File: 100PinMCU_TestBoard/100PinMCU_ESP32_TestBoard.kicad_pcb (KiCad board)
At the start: 4 copper layers, 117.6 x 50.6 mm, 120 parts, among them IC1 TCAN3413DR, IC2 TCAN3413DR, J1 ADC_Breakout, J10 SWD_PinHeader, J2 LogicAnalyzer_1, J3 CAN_1, J4 CAN_2, J5 LogicAnalyzer_2, J6 CAN_Breakout, J7 USB_C_Receptacle_USB2.0_16P, J8 SWD_Header_02x02, J9 USB_C_Receptacle_USB2.0_16P, SW1 BOOT Switch, SW2 RESET Button, U1 ESP32-C6-MINI-1, U2 MCP1826S, U3 STM32G491VET6, U4 TPS2117DRLR, Y1 Crystal

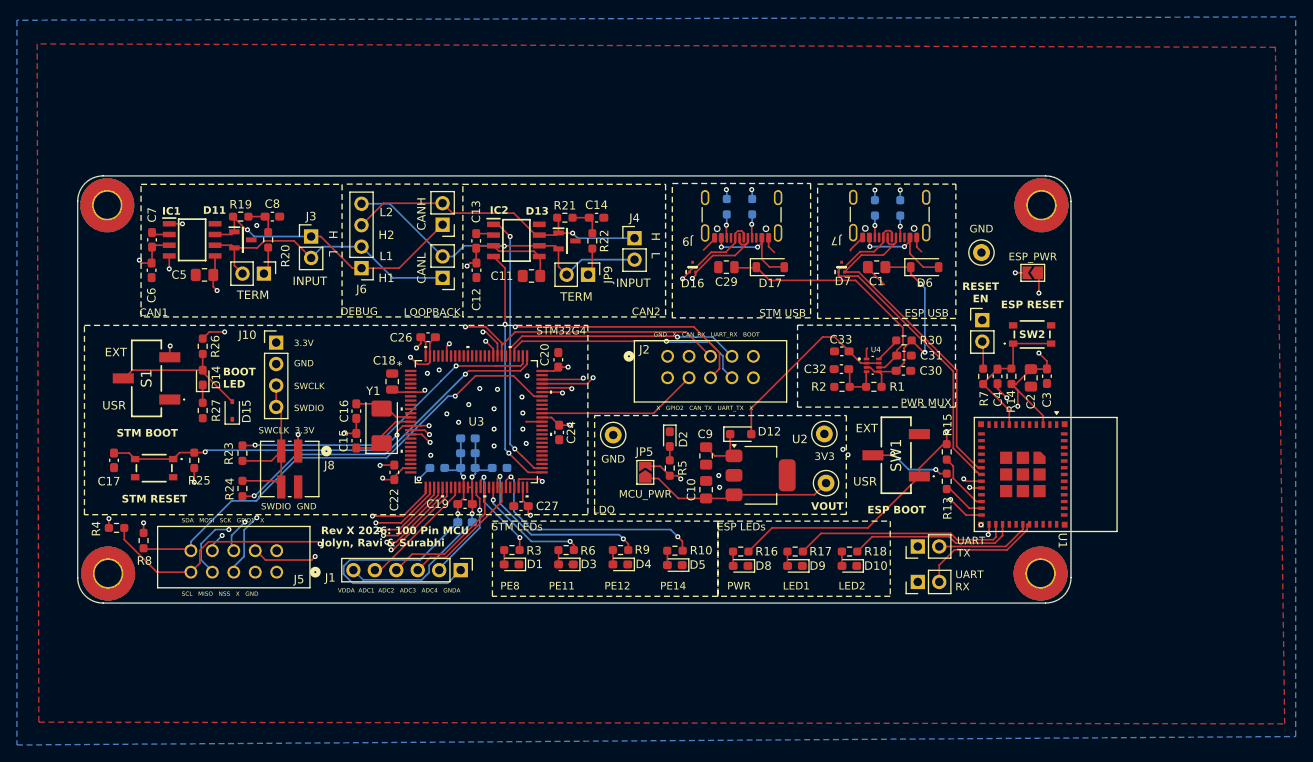
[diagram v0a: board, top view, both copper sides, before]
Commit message: oops my edge cuts were weird
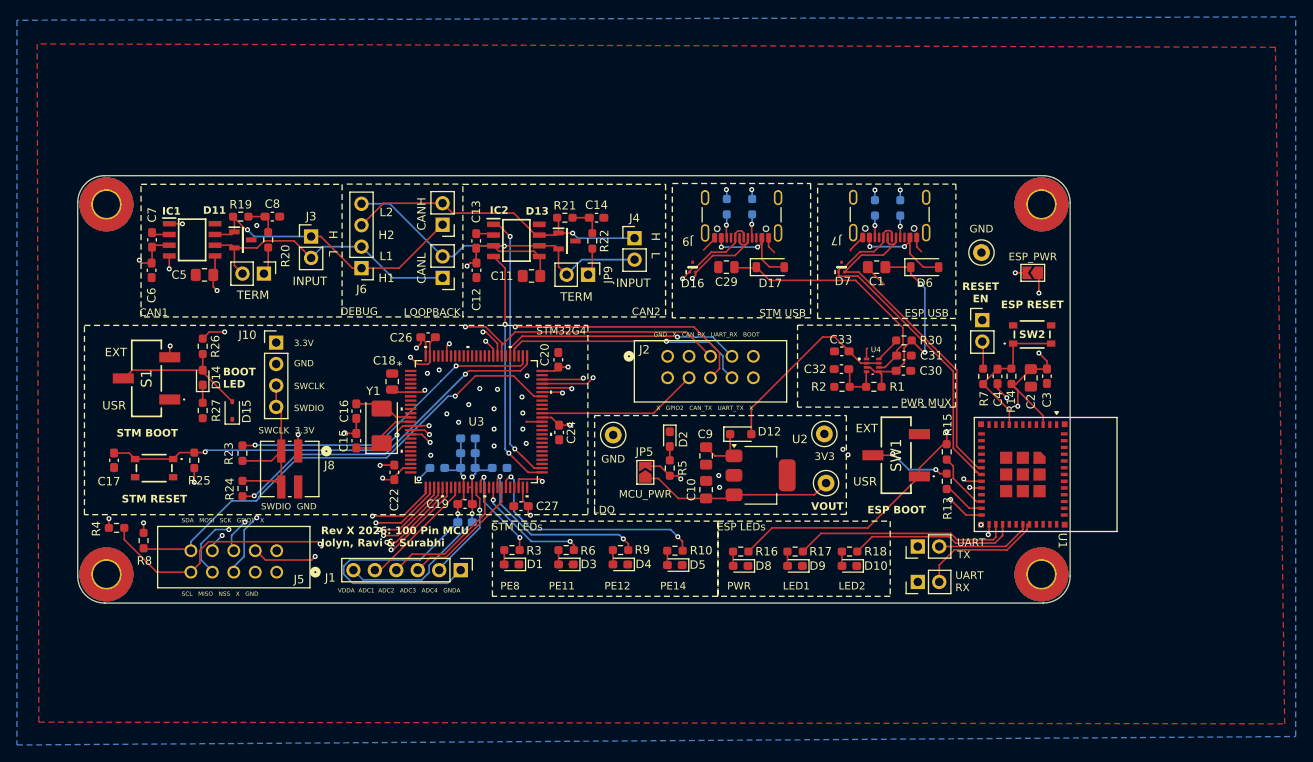
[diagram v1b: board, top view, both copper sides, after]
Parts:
- moved H1 0.22 mm to (87.6, 116.4)
- moved H4 0.14 mm to (198.3, 116.4)
- moved H2 0.14 mm to (87.6, 72.6)
- moved H3 0.10 mm to (198.3, 72.6)
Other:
- board size 117.6 x 50.6 mm -> 117.5 x 50.6 mm
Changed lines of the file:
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@@
 	(footprint "MountingHole:MountingHole_3.2mm_M3_Pad_TopBottom"
 		(layer "F.Cu")
-		(at 198.2 116.3)
+		(at 198.3 116.4)
 		(descr "Mounting Hole 3.2mm, M3, generated by kicad-footprint-generator mountinghole.py")
 		(tags "mountinghole M3")
@@
 	(footprint "MountingHole:MountingHole_3.2mm_M3_Pad_TopBottom"
 		(layer "F.Cu")
-		(at 198.3 72.7)
+		(at 198.3 72.6)
 		(descr "Mounting Hole 3.2mm, M3, generated by kicad-footprint-generator mountinghole.py")
 		(tags "mountinghole M3")
@@
 	(footprint "MountingHole:MountingHole_3.2mm_M3_Pad_TopBottom"
 		(layer "F.Cu")
-		(at 87.7 72.7)
+		(at 87.6 72.6)
 		(descr "Mounting Hole 3.2mm, M3, generated by kicad-footprint-generator mountinghole.py")
 		(tags "mountinghole M3")
@@
 	(footprint "MountingHole:MountingHole_3.2mm_M3_Pad_TopBottom"
 		(layer "F.Cu")
-		(at 87.8 116.3)
+		(at 87.6 116.4)
 		(descr "Mounting Hole 3.2mm, M3, generated by kicad-footprint-generator mountinghole.py")
 		(tags "mountinghole M3")
@@
 	)
 	(gr_line
-		(start 84.2 116.8)
-		(end 84.2 72.225)
+		(start 198.5 119.8)
+		(end 87.4 119.8)
 		(stroke
 			(width 0.05)
@@
 		(layer "Edge.Cuts")
 	)
-	(gr_arc
-		(start 201.8 116.8)
-		(mid 200.92132 118.92132)
-		(end 198.8 119.8)
+	(gr_line
+		(start 87.4 69.2)
+		(end 198.5 69.2)
 		(stroke
 			(width 0.05)
@@
 	)
 	(gr_arc
-		(start 84.2 72.225)
-		(mid 85.07868 70.10368)
-		(end 87.2 69.225)
+		(start 201.7 116.6)
+		(mid 200.762742 118.862742)
+		(end 198.5 119.8)
 		(stroke
 			(width 0.05)
@@
 	)
 	(gr_line
-		(start 201.8 72.225)
-		(end 201.8 116.8)
+		(start 84.2 116.6)
+		(end 84.2 72.4)
 		(stroke
 			(width 0.05)
@@
 		(layer "Edge.Cuts")
 	)
-	(gr_line
-		(start 198.8 119.8)
-		(end 87.2 119.8)
+	(gr_arc
+		(start 87.4 119.8)
+		(mid 85.137258 118.862742)
+		(end 84.2 116.6)
 		(stroke
 			(width 0.05)
@@
 		(layer "Edge.Cuts")
 	)
-	(gr_line
-		(start 87.2 69.225)
-		(end 198.8 69.225)
+	(gr_arc
+		(start 84.2 72.4)
+		(mid 85.137258 70.137258)
+		(end 87.4 69.2)
 		(stroke
 			(width 0.05)
@@
 	)
 	(gr_arc
-		(start 198.8 69.225)
-		(mid 200.92132 70.10368)
-		(end 201.8 72.225)
+		(start 198.5 69.2)
+		(mid 200.762742 70.137258)
+		(end 201.7 72.4)
 		(stroke
 			(width 0.05)
@@
 		(layer "Edge.Cuts")
 	)
-	(gr_arc
-		(start 87.2 119.8)
-		(mid 85.07868 118.92132)
-		(end 84.2 116.8)
+	(gr_line
+		(start 201.7 72.4)
+		(end 201.7 116.6)
 		(stroke
 			(width 0.05)
@@
 	)
 	(gr_text "UART\nTX"
-		(at 188.3 114.4 0)
+		(at 188.3 114.6 0)
 		(layer "F.SilkS" knockout)
 		(effects
@@
 	)
 	(gr_text "UART\nRX"
-		(at 188.1 118.4 0)
+		(at 188.1 118.5 0)
 		(layer "F.SilkS" knockout)
 		(effects
@@
 		)
 	)
+	(dimension
+		(type orthogonal)
+		(layer "Dwgs.User")
+		(pts
+			(xy 84.2 75.9) (xy 201.8 76)
+		)
+		(height -10.8)
+		(orientation 0)
+		(format
+			(prefix "")
+			(suffix "")
+			(units 3)
+			(units_format 0)
+			(precision 4)
+			(suppress_zeroes yes)
+		)
+		(style
+			(thickness 0.1)
+			(arrow_length 1.27)
+			(text_position_mode 0)
+			(arrow_direction outward)
+			(extension_height 0.58642)
+			(extension_offset 0.5)
+			(keep_text_aligned yes)
+		)
+		(gr_text "117.6"
+			(at 143 63.95 0)
+			(layer "Dwgs.User")
+			(effects
+				(font
+					(size 1 1)
+					(thickness 0.15)
+				)
+			)
+		)
+	)
+	(dimension
+		(type orthogonal)
+		(layer "Dwgs.User")
+		(pts
+			(xy 91.7 69.2) (xy 91.5 119.8)
+		)
+		(height -9)
+		(orientation 1)
+		(format
+			(prefix "")
+			(suffix "")
+			(units 3)
+			(units_format 0)
+			(precision 4)
+			(suppress_zeroes yes)
+		)
+		(style
+			(thickness 0.1)
+			(arrow_length 1.27)
+			(text_position_mode 0)
+			(arrow_direction outward)
+			(extension_height 0.58642)
+			(extension_offset 0.5)
+			(keep_text_aligned yes)
+		)
+		(gr_text "50.6"
+			(at 81.55 94.5 90)
+			(layer "Dwgs.User")
+			(effects
+				(font
+					(size 1 1)
+					(thickness 0.15)
+				)
+			)
+		)
+	)
